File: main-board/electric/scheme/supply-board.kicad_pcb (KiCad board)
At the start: 2 copper layers, 85 x 56 mm, 139 parts, among them K1 CONN_3, P1 PWR-IN, P10 TST, P11 TST, P12 PWR-IN, P13 CONN_4, P14 PWR-IN, P16 TST, P17 TST, P18 TST, P19 TST, P2 PWR-IN, P3 CONN_4, P4 CONN_10, P5 PWR-IN, P6 TST, P7 TST, P8 TST, P9 CONN_3X2, Q1 BC847, Q10 MOS_N, Q11 MOS_P, Q12 MOS_P, Q2 BC847, Q3 BC847, Q4 MOS_P, Q5 BC847, Q6 BC857, Q7 BC847, Q8 BC857, Q9 BC847, U1 NCP3063, U2 L293, U3 MINI-USB-B, X1 8MHz

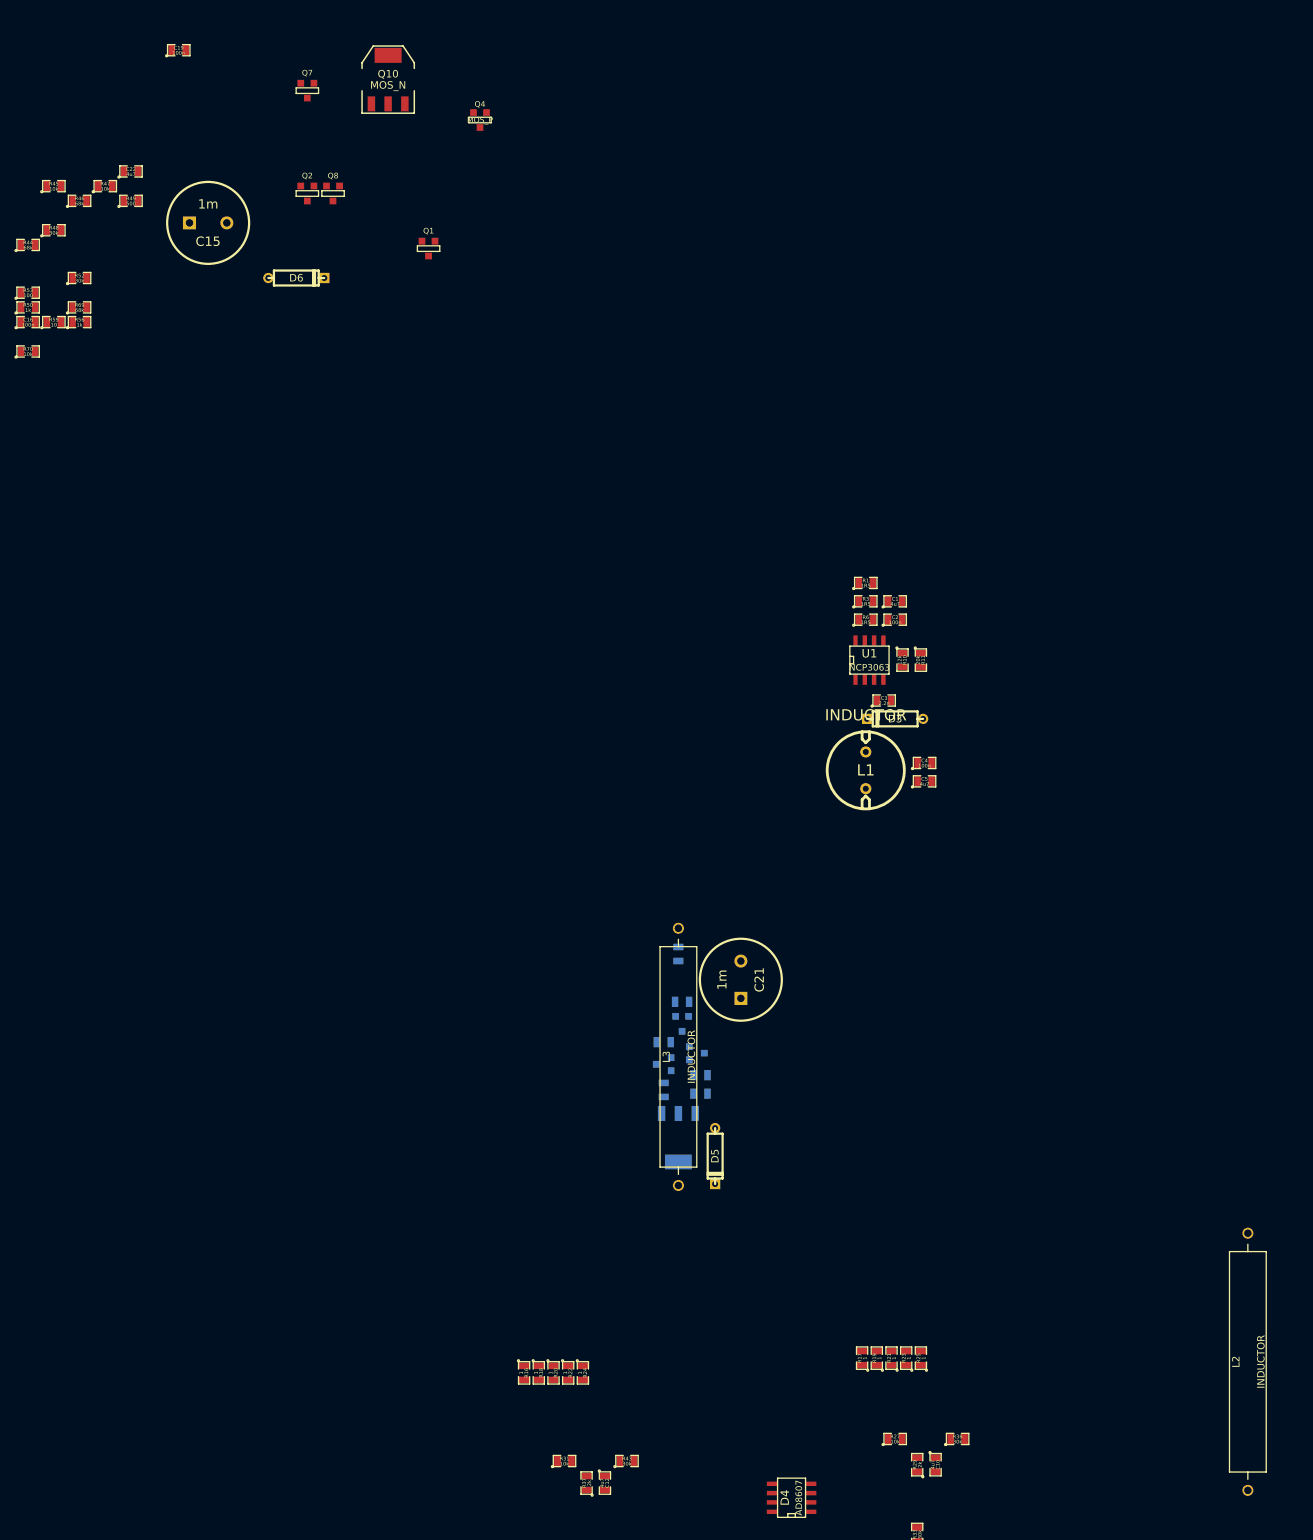
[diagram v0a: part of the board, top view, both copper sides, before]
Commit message: Placing components...
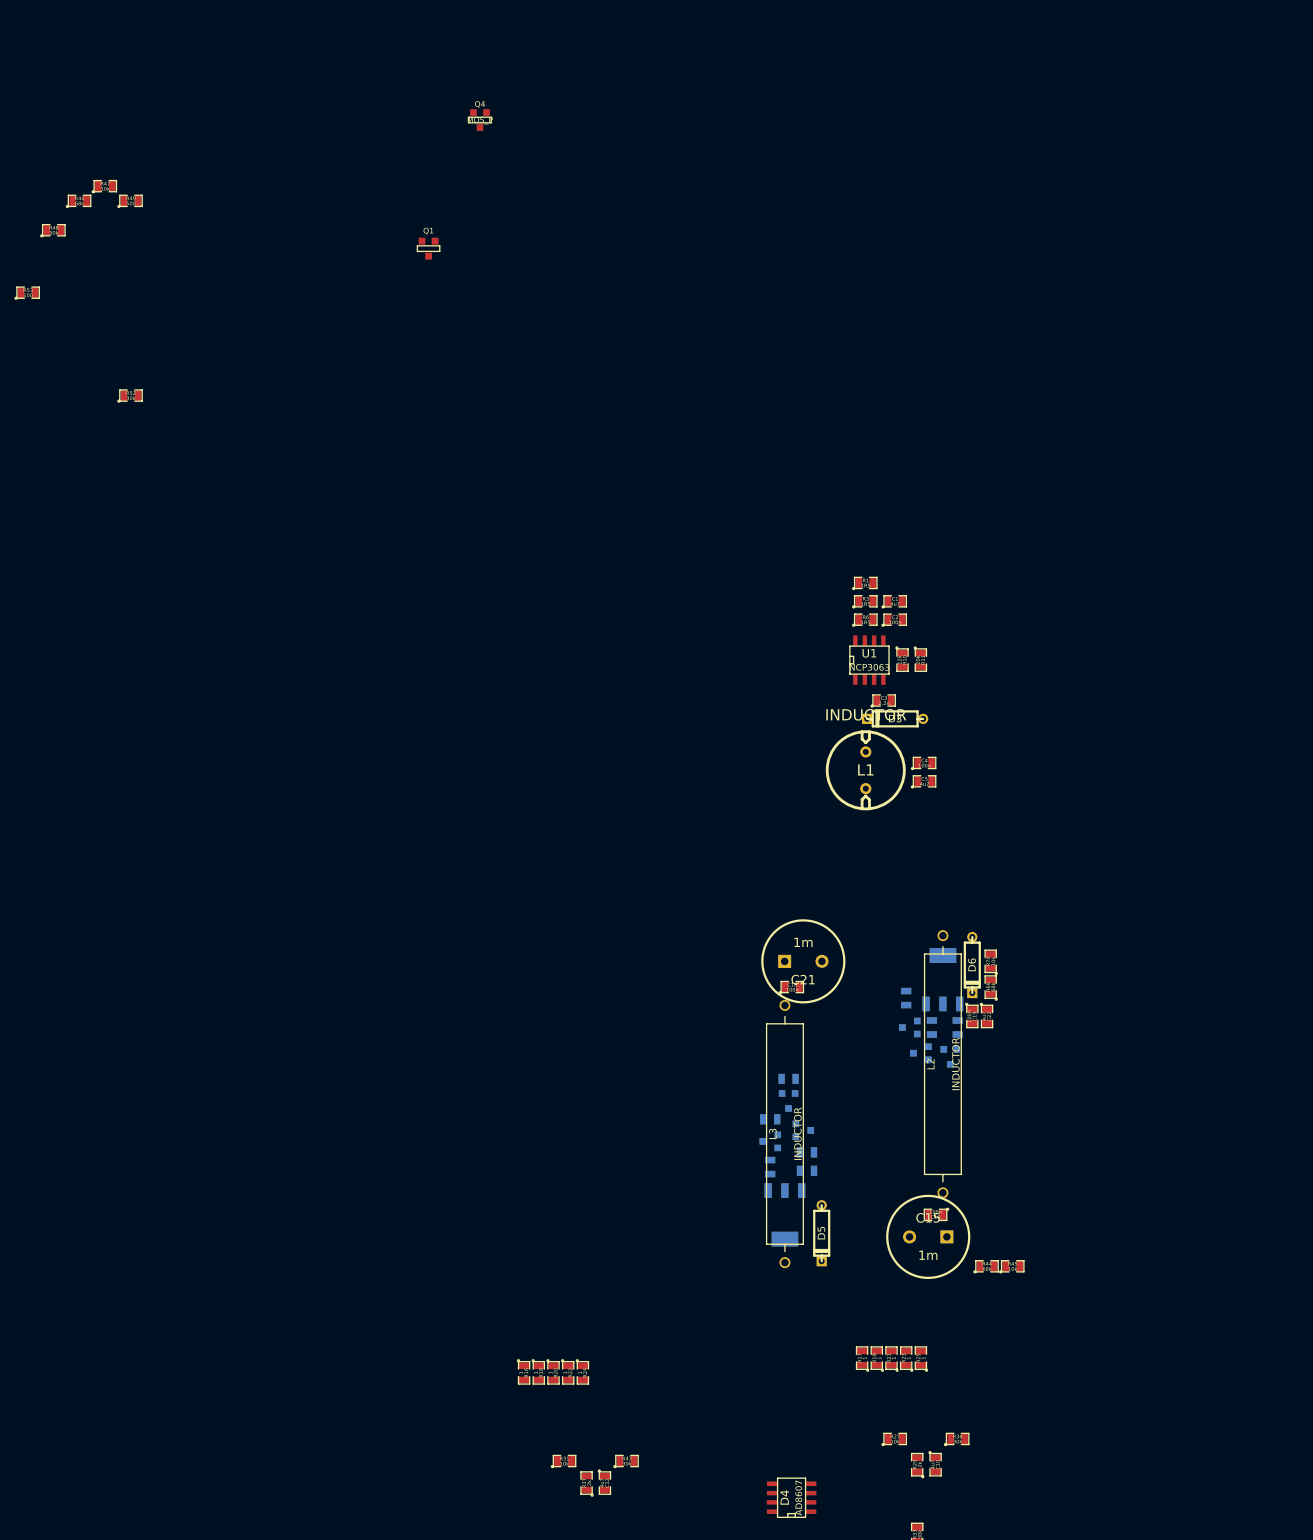
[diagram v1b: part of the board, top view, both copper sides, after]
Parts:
- C18: moved to F.Cu
- Q10, Q2, Q7, Q8, R50, R56, R59: moved to B.Cu
- moved R45 196.6 mm to (91.0, 141.5)
- moved R44 190.7 mm to (87.5, 141.5)
- moved C16 173.2 mm to (80.5, 134.5), turned to 180 degrees
- moved C19 170.2 mm to (85.5, 107.5), turned to 270 degrees
- moved C15 169.3 mm to (79.5, 137.5), turned to 180 degrees
- moved C22 163.7 mm to (87.5, 107.5), turned to 270 degrees
- moved R59 156.0 mm to (83.5, 109.0), turned to 90 degrees
- moved Q7 155.3 mm to (78.5, 112.5), turned to 90 degrees
- moved R70 155.1 mm to (88.0, 100.0), turned to 90 degrees
- moved R69 154.7 mm to (88.0, 103.5), turned to 90 degrees
- moved R50 152.0 mm to (76.5, 105.0), turned to 90 degrees
- moved R56 150.6 mm to (80.0, 109.0), turned to 90 degrees
- moved Q8 144.4 mm to (82.5, 113.0), turned to 180 degrees
- moved Q10 143.9 mm to (81.5, 102.5), turned to 180 degrees
- moved Q2 140.0 mm to (77.0, 109.0), turned to 90 degrees
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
